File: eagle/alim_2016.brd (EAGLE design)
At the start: 93.1 x 50.4 mm, 57 parts, among them J1 AVR_SPI_PRG_6PTH, J2 AVR_SPI_PRG_6PTH, U1 3.3V, U2 LM2678S-5.0, U4 LM2596S-ADJ, U5 ATTINY85-20SU, U6 ATMEGA328P_TQFP

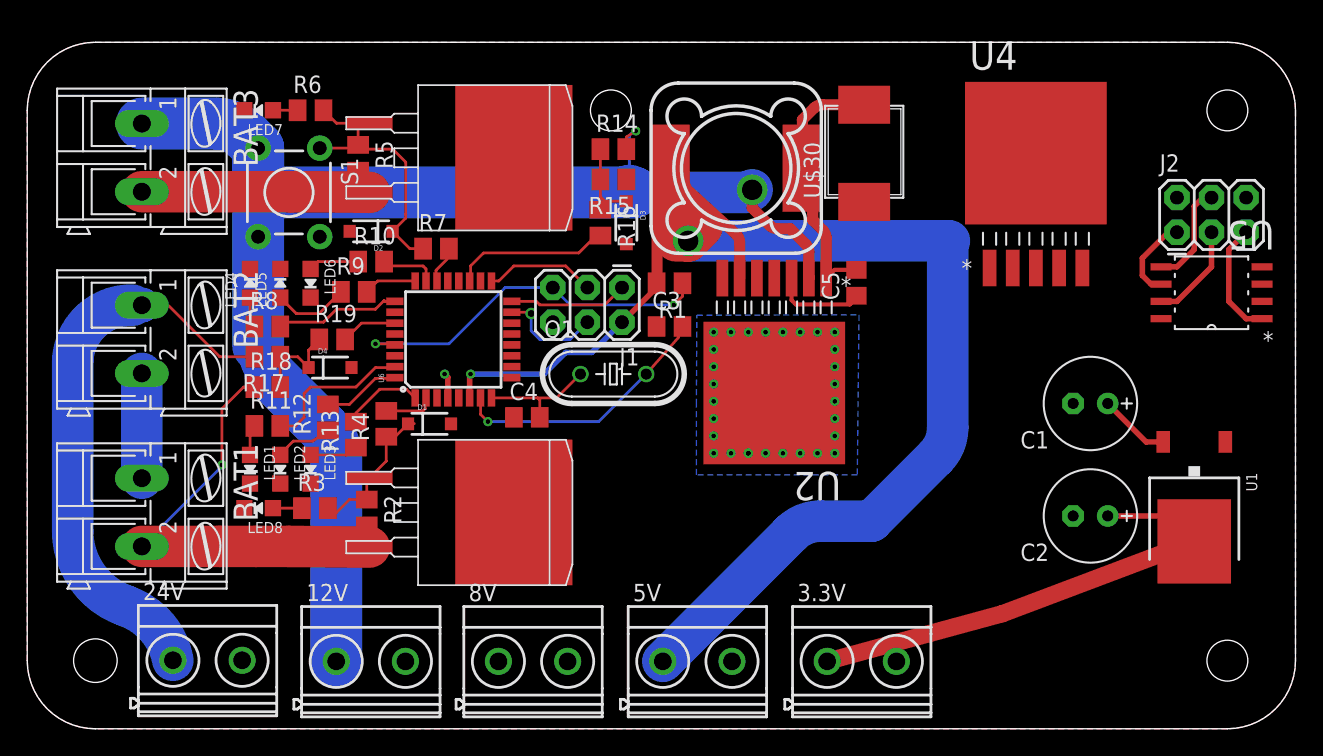
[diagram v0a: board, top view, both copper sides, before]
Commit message: neater
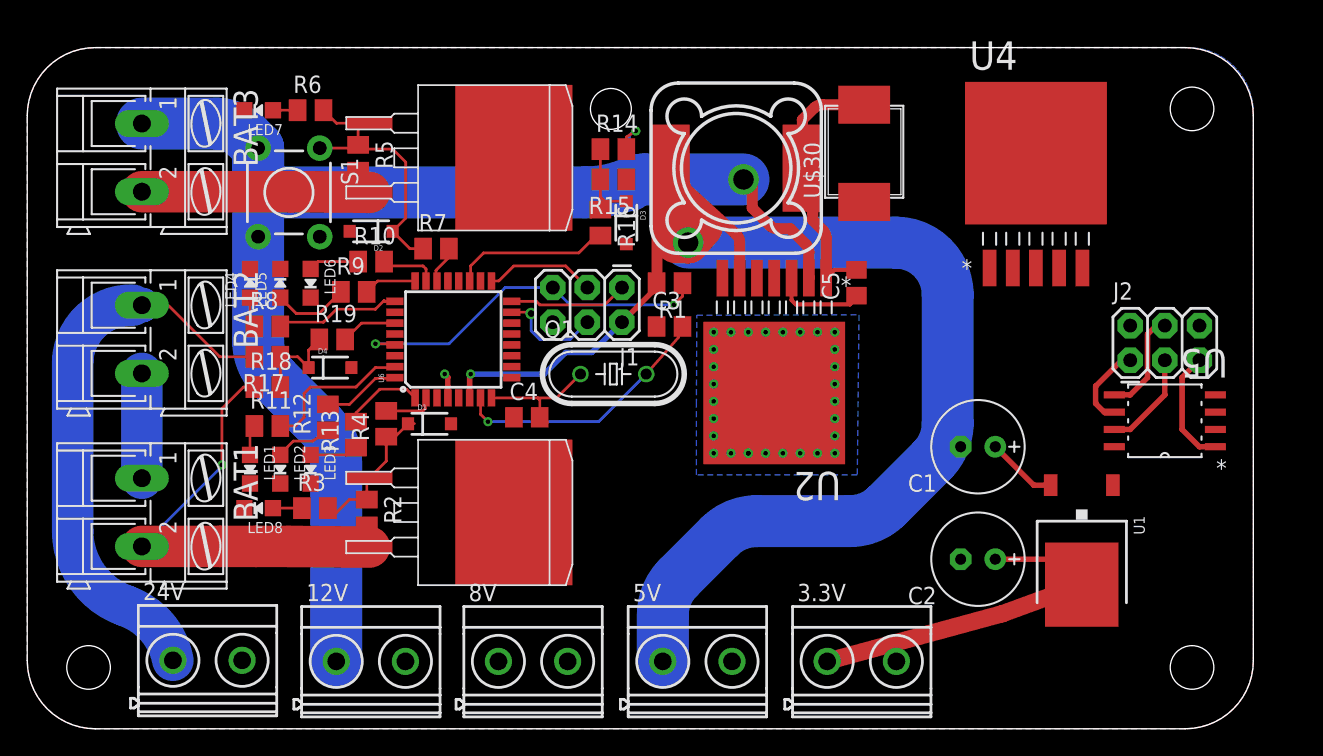
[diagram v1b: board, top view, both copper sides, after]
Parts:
- moved U5 10.0 mm to (83.5, 22.6)
- moved J2 10.0 mm to (81.0, 27.1)
- moved U1 8.84 mm to (77.4, 13.1)
- moved C1 8.84 mm to (69.8, 20.7)
- moved C2 8.84 mm to (69.8, 12.4)
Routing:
- net N$1: track 35.5 -> 26.7 mm
- net 12V: track 104.5 -> 105.5 mm
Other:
- board size 93.1 x 50.4 mm -> 90 x 50 mm
